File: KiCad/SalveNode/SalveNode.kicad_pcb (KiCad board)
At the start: 2 copper layers, 42.6 x 31.1 mm, 19 parts, among them IC1 DS89C21TMX_NOPB, IC2 TMP75AQDGKRQ1, IC3 ATMEGA328PB-AN, IC4 VEML7700-TR, J1 Screw_Terminal_01x06, J2 Screw_Terminal_01x06, Y1 Crystal

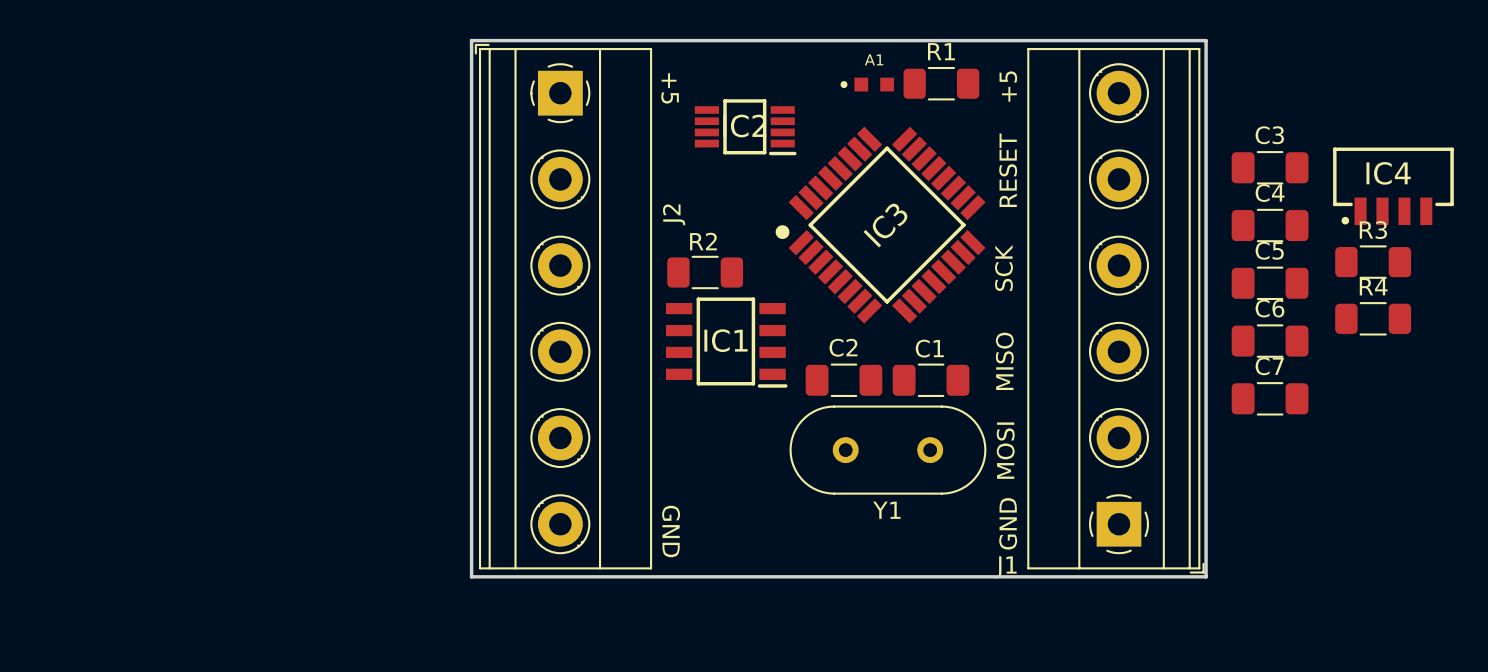
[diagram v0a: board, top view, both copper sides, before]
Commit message: PCB Complete
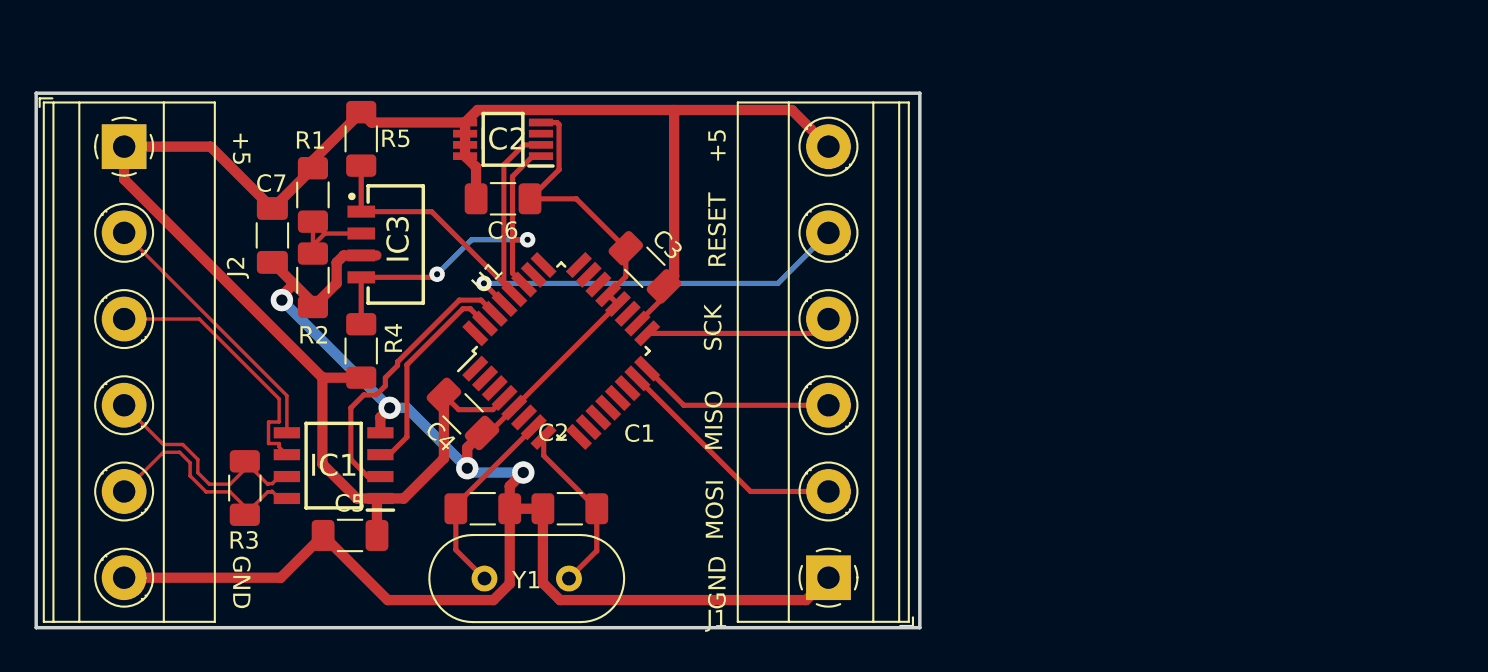
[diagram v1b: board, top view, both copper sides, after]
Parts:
- removed A1: ALS-PT19-315C_L177_TR8, SimbolosSnapEDA:XDCR_ALS-PT19-315C_L177_TR8
- removed the IC3 at (166.6, 47.6)
- added R2: R, Resistor_SMD:R_1206_3216Metric_Pad1.30x1.75mm_HandSolder, F.Cu at (133.3, 50.9)
- added U1: ATmega328PB-A, Package_QFP:TQFP-32_7x7mm_P0.8mm, F.Cu at (147.7, 55.0)
- R1: value 10k -> R
- moved R5 59.6 mm to (136.1, 42.6), turned to 90 degrees
- moved R4 58.9 mm to (136.1, 55.0), turned to 90 degrees
- moved C7 58.6 mm to (130.9, 48.2), turned to 90 degrees
- moved IC3 56.1 mm to (136.5, 45.4), turned to -90 degrees
- moved C5 55.3 mm to (135.4, 65.7)
- moved C4 48.1 mm to (142.0, 58.6), turned to 135 degrees
- moved C6 45.2 mm to (144.3, 46.1), turned to 180 degrees
- moved R1 37.0 mm to (133.3, 45.9), turned to -90 degrees
- moved C3 36.7 mm to (152.6, 50.1), turned to -45 degrees
- moved R3 29.5 mm to (129.3, 62.9), turned to 90 degrees
- moved J2 25.5 mm to (122.3, 43.1)
- moved IC1 23.9 mm to (134.5, 61.6)
- moved C1 22.2 mm to (148.2, 64.1)
- moved Y1 22.2 mm to (148.2, 68.2)
- moved C2 22.2 mm to (143.2, 64.1)
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- renumbered IC4 to IC3, R2 to R3, R3 to R4, R4 to R5
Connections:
- IC2 pad 5: Earth -> +5V
- IC2 pad 6: Earth -> +5V
- IC2 pad 7: Earth -> +5V
- IC3 pad 2: Net-(IC4-VDD) -> Net-(IC3-VDD)
- R1 pad 1: /LIGHT_IN -> +5V
- R1 pad 2: Earth -> Net-(IC3-VDD)
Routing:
- net Earth: track 0.00 -> 116.2 mm, vias 0 -> 4
- net +5V: track 0.00 -> 108.6 mm
- net /SCL: track 0.00 -> 23.9 mm
- net /RESET: track 0.00 -> 22.9 mm, vias 0 -> 1
- net /SDA: track 0.00 -> 22.8 mm, vias 0 -> 2
- net /RX: track 0.00 -> 17.3 mm
- net /D0+: track 0.00 -> 15.6 mm
- net /D0-: track 0.00 -> 15.5 mm
- net /MOSI: track 0.00 -> 13.8 mm
- net /RI+: track 0.00 -> 13.3 mm
- net /RI-: track 0.00 -> 13.3 mm
- net /TX: track 0.00 -> 12.4 mm
- net /MISO: track 0.00 -> 11.4 mm
- net /XTAL1: track 0.00 -> 11.4 mm
- net /SCK: track 0.00 -> 10.9 mm
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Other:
- board size 42.6 x 31.1 mm -> 51.2 x 31 mm
